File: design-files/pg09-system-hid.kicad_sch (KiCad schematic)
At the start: 3 parts, among them J1101 PS/2 Keyboard, J1102 SNES-Controller-Socket, J1103 SNES-Controller-Socket

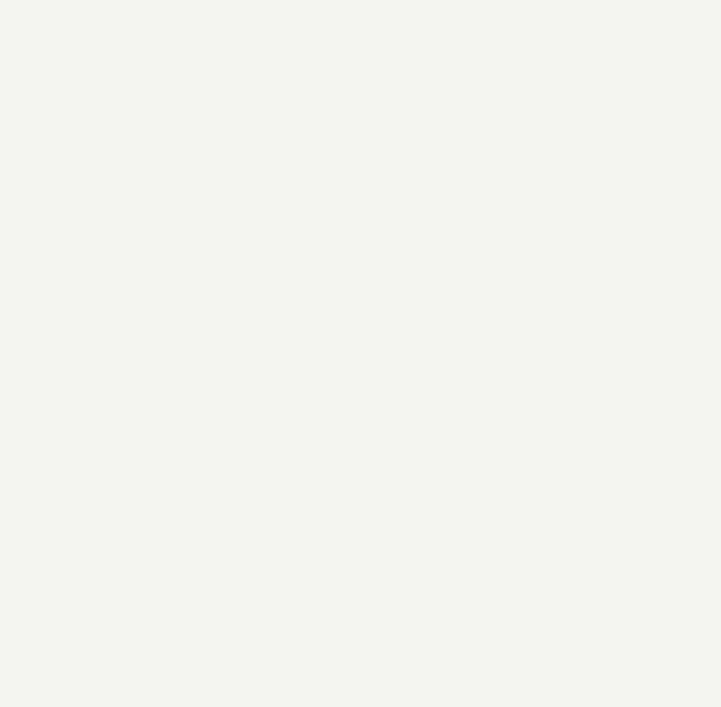
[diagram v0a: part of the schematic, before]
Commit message: Add VERA module connector that will house video.
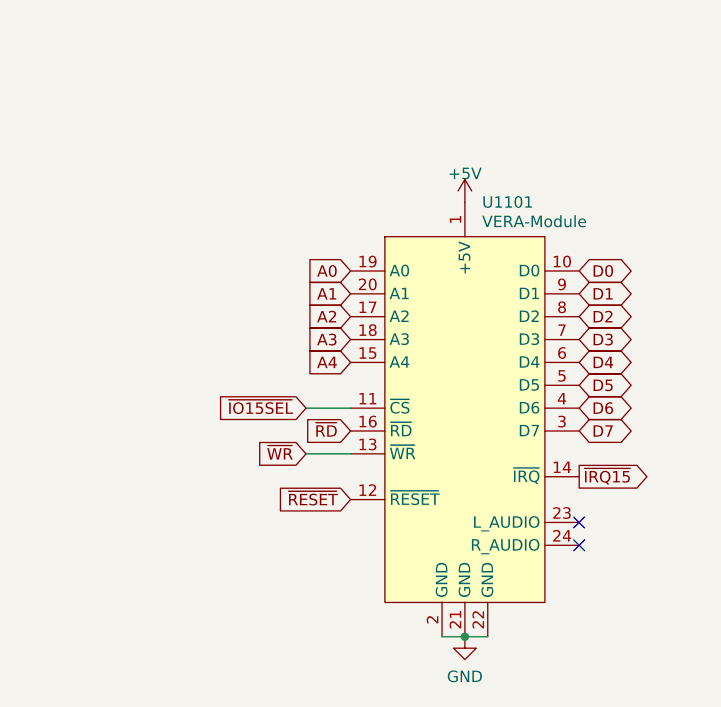
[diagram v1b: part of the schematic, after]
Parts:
- added U1101: VERA-Module, jrt-Connectors:VERA-Module, symbol jrt-ICs:VERA-Module
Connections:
- new net +5V: U1101.1 (+5V)
- new net A0: U1101.19 (A0)
- new net A1: U1101.20 (A1)
- new net A2: U1101.17 (A2)
- new net A3: U1101.18 (A3)
- new net A4: U1101.15 (A4)
- new net D0: U1101.10 (D0)
- new net D1: U1101.9 (D1)
- new net D2: U1101.8 (D2)
- new net D3: U1101.7 (D3)
- new net D4: U1101.6 (D4)
- new net D5: U1101.5 (D5)
- new net D6: U1101.4 (D6)
- new net D7: U1101.3 (D7)
- new net GND: U1101.2 (GND), U1101.21 (GND), U1101.22 (GND)
- new net ~{IO15SEL}: U1101.11 (~{CS})
- new net ~{IRQ15}: U1101.14 (~{IRQ})
- new net ~{RD}: U1101.16 (~{RD})
- new net ~{RESET}: U1101.12 (~{RESET})
- new net ~{WR}: U1101.13 (~{WR})
- no-connect marks 20 -> 22
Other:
- company: Copyright (c) 2022-2023 Jason R. Thorpe. See LICENSE. -> Copyright (c) 2022-2024 Jason R. Thorpe. See LICENSE.
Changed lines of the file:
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@@
     (title "6809 Playground system board")
     (date "2023-07-16")
-    (company "Copyright (c) 2022-2023 Jason R. Thorpe. See LICENSE.")
+    (company "Copyright (c) 2022-2024 Jason R. Thorpe. See LICENSE.")
+  )
+  (junction (at 202.565 116.967) (diameter 0) (color 0 0 0 0)
   )
   (no_connect (at 90.424 78.232))
@@
   (no_connect (at 38.1 75.438))
   (no_connect (at 90.424 103.886))
+  (no_connect (at 215.265 104.267))
   (no_connect (at 90.424 80.772))
+  (no_connect (at 215.265 106.807))
+  (wire (pts (xy 184.912 91.567) (xy 189.865 91.567))
+    (stroke (width 0) (type default))
+  )
+  (wire (pts (xy 200.025 116.967) (xy 202.565 116.967))
+    (stroke (width 0) (type default))
+  )
+  (wire (pts (xy 184.912 96.647) (xy 189.865 96.647))
+    (stroke (width 0) (type default))
+  )
+  (wire (pts (xy 202.565 116.967) (xy 205.105 116.967))
+    (stroke (width 0) (type default))
+  )
   (text "Human Interface Devices" (at 121.92 22.606 0)
     (effects (font (size 2.54 2.54) (thickness 0.254) bold italic) (justify left bottom))
+  )
+  (global_label "~{RD}" (shape input) (at 189.865 94.107 180) (fields_autoplaced)
+    (effects (font (size 1.27 1.27)) (justify right))
+    (property "Intersheetrefs" "${INTERSHEET_REFS}" (at 184.4192 94.107 0)
+      (effects (font (size 1.27 1.27)) (justify right) hide)
+    )
+  )
+  (global_label "A4" (shape input) (at 189.865 86.487 180) (fields_autoplaced)
+    (effects (font (size 1.27 1.27)) (justify right))
+    (property "Intersheetrefs" "${INTERSHEET_REFS}" (at 184.6611 86.487 0)
+      (effects (font (size 1.27 1.27)) (justify right) hide)
+    )
+  )
+  (global_label "D1" (shape bidirectional) (at 215.265 78.867 0) (fields_autoplaced)
+    (effects (font (size 1.27 1.27)) (justify left))
+    (property "Intersheetrefs" "${INTERSHEET_REFS}" (at 221.7616 78.867 0)
+      (effects (font (size 1.27 1.27)) (justify left) hide)
+    )
+  )
+  (global_label "~{WR}" (shape input) (at 184.912 96.647 180) (fields_autoplaced)
+    (effects (font (size 1.27 1.27)) (justify right))
+    (property "Intersheetrefs" "${INTERSHEET_REFS}" (at 179.2848 96.647 0)
+      (effects (font (size 1.27 1.27)) (justify right) hide)
+    )
+  )
+  (global_label "A3" (shape input) (at 189.865 83.947 180) (fields_autoplaced)
+    (effects (font (size 1.27 1.27)) (justify right))
+    (property "Intersheetrefs" "${INTERSHEET_REFS}" (at 184.6611 83.947 0)
+      (effects (font (size 1.27 1.27)) (justify right) hide)
+    )
+  )
+  (global_label "D7" (shape bidirectional) (at 215.265 94.107 0) (fields_autoplaced)
+    (effects (font (size 1.27 1.27)) (justify left))
+    (property "Intersheetrefs" "${INTERSHEET_REFS}" (at 221.7616 94.107 0)
+      (effects (font (size 1.27 1.27)) (justify left) hide)
+    )
+  )
+  (global_label "A0" (shape input) (at 189.865 76.327 180) (fields_autoplaced)
+    (effects (font (size 1.27 1.27)) (justify right))
+    (property "Intersheetrefs" "${INTERSHEET_REFS}" (at 184.6611 76.327 0)
+      (effects (font (size 1.27 1.27)) (justify right) hide)
+    )
+  )
+  (global_label "D6" (shape bidirectional) (at 215.265 91.567 0) (fields_autoplaced)
+    (effects (font (size 1.27 1.27)) (justify left))
+    (property "Intersheetrefs" "${INTERSHEET_REFS}" (at 221.7616 91.567 0)
+      (effects (font (size 1.27 1.27)) (justify left) hide)
+    )
+  )
+  (global_label "~{RESET}" (shape input) (at 189.865 101.727 180) (fields_autoplaced)
+    (effects (font (size 1.27 1.27)) (justify right))
+    (property "Intersheetrefs" "${INTERSHEET_REFS}" (at 181.2141 101.727 0)
+      (effects (font (size 1.27 1.27)) (justify right) hide)
+    )
+  )
+  (global_label "D5" (shape bidirectional) (at 215.265 89.027 0) (fields_autoplaced)
+    (effects (font (size 1.27 1.27)) (justify left))
+    (property "Intersheetrefs" "${INTERSHEET_REFS}" (at 221.7616 89.027 0)
+      (effects (font (size 1.27 1.27)) (justify left) hide)
+    )
+  )
+  (global_label "D0" (shape bidirectional) (at 215.265 76.327 0) (fields_autoplaced)
+    (effects (font (size 1.27 1.27)) (justify left))
+    (property "Intersheetrefs" "${INTERSHEET_REFS}" (at 221.7616 76.327 0)
+      (effects (font (size 1.27 1.27)) (justify left) hide)
+    )
+  )
+  (global_label "A2" (shape input) (at 189.865 81.407 180) (fields_autoplaced)
+    (effects (font (size 1.27 1.27)) (justify right))
+    (property "Intersheetrefs" "${INTERSHEET_REFS}" (at 184.6611 81.407 0)
+      (effects (font (size 1.27 1.27)) (justify right) hide)
+    )
+  )
+  (global_label "~{IO15SEL}" (shape input) (at 184.912 91.567 180) (fields_autoplaced)
+    (effects (font (size 1.27 1.27)) (justify right))
+    (property "Intersheetrefs" "${INTERSHEET_REFS}" (at 174.2653 91.567 0)
+      (effects (font (size 1.27 1.27)) (justify right) hide)
+    )
+  )
+  (global_label "D3" (shape bidirectional) (at 215.265 83.947 0) (fields_autoplaced)
+    (effects (font (size 1.27 1.27)) (justify left))
+    (property "Intersheetrefs" "${INTERSHEET_REFS}" (at 221.7616 83.947 0)
+      (effects (font (size 1.27 1.27)) (justify left) hide)
+    )
+  )
+  (global_label "D4" (shape bidirectional) (at 215.265 86.487 0) (fields_autoplaced)
+    (effects (font (size 1.27 1.27)) (justify left))
+    (property "Intersheetrefs" "${INTERSHEET_REFS}" (at 221.7616 86.487 0)
+      (effects (font (size 1.27 1.27)) (justify left) hide)
+    )
+  )
+  (global_label "~{IRQ15}" (shape output) (at 215.265 99.187 0) (fields_autoplaced)
+    (effects (font (size 1.27 1.27)) (justify left))
+    (property "Intersheetrefs" "${INTERSHEET_REFS}" (at 223.7951 99.187 0)
+      (effects (font (size 1.27 1.27)) (justify left) hide)
+    )
+  )
+  (global_label "D2" (shape bidirectional) (at 215.265 81.407 0) (fields_autoplaced)
+    (effects (font (size 1.27 1.27)) (justify left))
+    (property "Intersheetrefs" "${INTERSHEET_REFS}" (at 221.7616 81.407 0)
+      (effects (font (size 1.27 1.27)) (justify left) hide)
+    )
+  )
+  (global_label "A1" (shape input) (at 189.865 78.867 180) (fields_autoplaced)
+    (effects (font (size 1.27 1.27)) (justify right))
+    (property "Intersheetrefs" "${INTERSHEET_REFS}" (at 184.6611 78.867 0)
+      (effects (font (size 1.27 1.27)) (justify right) hide)
+    )
+  )
+  (symbol (lib_id "jrt-ICs:VERA-Module") (at 202.565 91.567 0) (unit 1)
+    (in_bom yes) (on_board yes) (dnp no)
+    (property "Reference" "U1101" (at 204.47 68.707 0)
+      (effects (font (size 1.27 1.27)) (justify left))
+    )
+    (property "Value" "VERA-Module" (at 204.47 70.866 0)
+      (effects (font (size 1.27 1.27)) (justify left))
+    )
+    (property "Footprint" "jrt-Connectors:VERA-Module" (at 203.835 86.487 0)
+      (effects (font (size 1.27 1.27)) hide)
+    )
+    (property "Datasheet" "https://github.com/X16Community/vera-module/tree/main" (at 203.835 86.487 0)
+      (effects (font (size 1.27 1.27)) hide)
+    )
+    (property "Sim.Enable" "0" (at 202.565 91.567 0)
+      (effects (font (size 1.27 1.27)) hide)
+    )
+    (pin "1")
+    (pin "10")
+    (pin "11")
+    (pin "12")
+    (pin "13")
+    (pin "14")
+    (pin "15")
+    (pin "16")
+    (pin "17")
+    (pin "18")
+    (pin "19")
+    (pin "2")
+    (pin "20")
+    (pin "21")
+    (pin "22")
+    (pin "23")
+    (pin "24")
+    (pin "3")
+    (pin "4")
+    (pin "5")
+    (pin "6")
+    (pin "7")
+    (pin "8")
+    (pin "9")
+    (instances
+      (project "pg09-system"
+        (path "/44572023-3621-4b3a-bd53-c3b2b3f42871/2aac33c7-62da-4c06-b1d4-3434ee198b44"
+          (reference "U1101") (unit 1)
+        )
+      )
+    )
+  )
+  (symbol (lib_id "power:+5V") (at 202.565 68.707 0) (unit 1)
+    (in_bom yes) (on_board yes) (dnp no) (fields_autoplaced)
+    (property "Reference" "#PWR01101" (at 202.565 72.517 0)
+      (effects (font (size 1.27 1.27)) hide)
+    )
+    (property "Value" "+5V" (at 202.565 65.532 0)
+      (effects (font (size 1.27 1.27)))
+    )
+    (property "Footprint" "" (at 202.565 68.707 0)
+      (effects (font (size 1.27 1.27)) hide)
+    )
+    (property "Datasheet" "" (at 202.565 68.707 0)
+      (effects (font (size 1.27 1.27)) hide)
+    )
+    (pin "1")
+    (instances
+      (project "pg09-system"
+        (path "/44572023-3621-4b3a-bd53-c3b2b3f42871/2aac33c7-62da-4c06-b1d4-3434ee198b44"
+          (reference "#PWR01101") (unit 1)
+        )
+      )
+    )
   )
   (symbol (lib_id "jrt-SNES:SNES-Controller-Socket") (at 99.314 65.532 0) (unit 1)
@@
         )
       )
+    )
+  )
+  (symbol (lib_id "power:GND") (at 202.565 116.967 0) (unit 1)
+    (in_bom yes) (on_board yes) (dnp no) (fields_autoplaced)
+    (property "Reference" "#PWR01102" (at 202.565 123.317 0)
+      (effects (font (size 1.27 1.27)) hide)
+    )
+    (property "Value" "GND" (at 202.565 121.412 0)
+      (effects (font (size 1.27 1.27)))
+    )
+    (property "Footprint" "" (at 202.565 116.967 0)
+      (effects (font (size 1.27 1.27)) hide)
+    )
+    (property "Datasheet" "" (at 202.565 116.967 0)
+      (effects (font (size 1.27 1.27)) hide)
+    )
+    (pin "1")
+    (instances
+      (project "pg09-system"
+        (path "/44572023-3621-4b3a-bd53-c3b2b3f42871/2aac33c7-62da-4c06-b1d4-3434ee198b44"
+          (reference "#PWR01102") (unit 1)
+        )
+      )
